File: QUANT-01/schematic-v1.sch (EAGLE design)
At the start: 1 part, among them U1 MCP4725

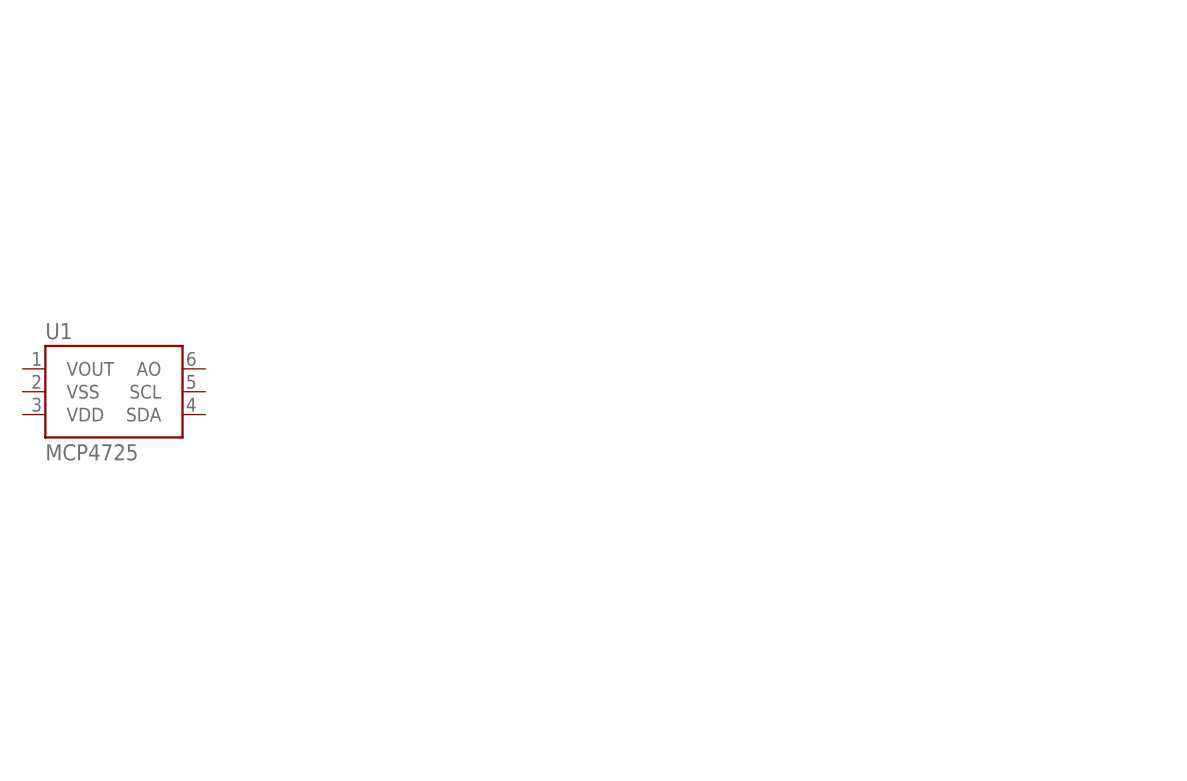
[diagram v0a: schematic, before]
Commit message: kind of got the quantization of Vin working.
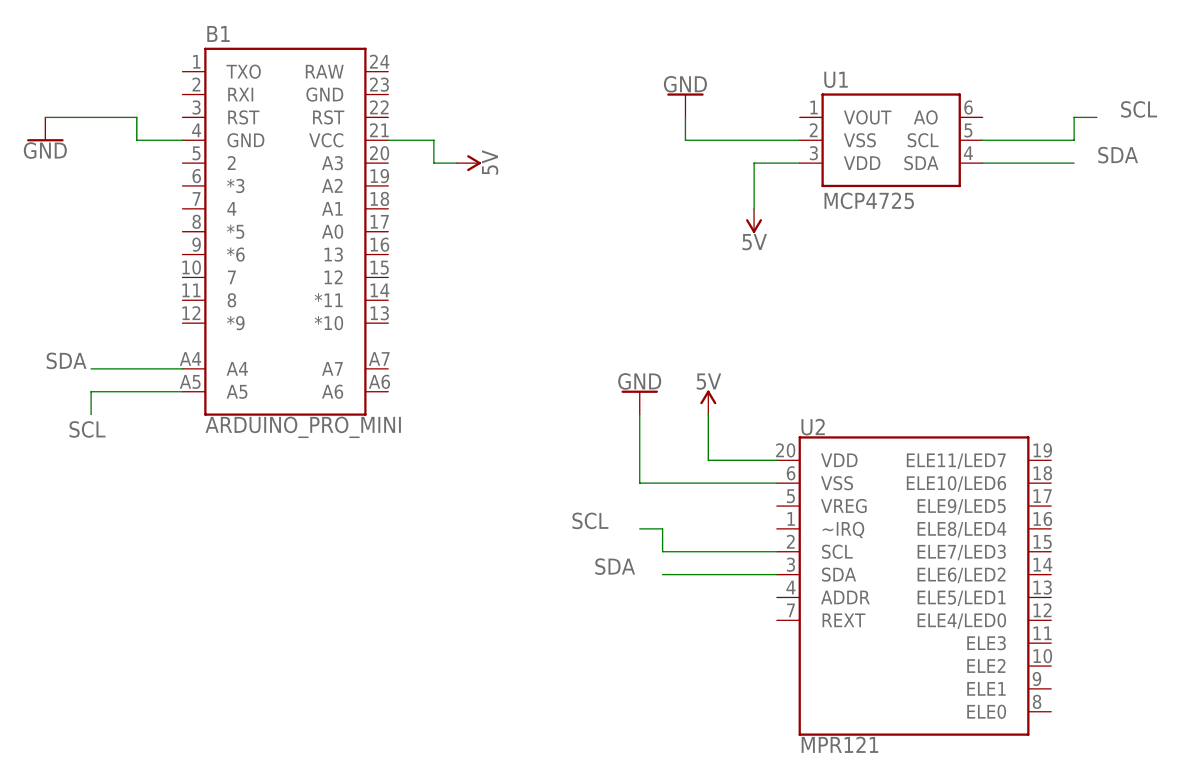
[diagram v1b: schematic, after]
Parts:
- added B1: ARDUINO_PRO_MINI, SparkFun-Boards:ARDUINO_PRO_MINI
- added U2: MPR121, SparkFun-Sensors:MPR121
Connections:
- new net 5V: B1.VCC, U1.VDD, U2.VDD
- new net GND: B1.GND, U1.VSS, U2.VSS
- new net SCL: B1.A5, U1.SCL, U2.SCL
- new net SDA: B1.A4, U1.SDA, U2.SDA
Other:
- moved on the sheet: U1
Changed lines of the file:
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@@
 <layer number="230" name="230bmp" color="7" fill="1" visible="yes" active="yes"/>
 <layer number="231" name="231bmp" color="7" fill="1" visible="yes" active="yes"/>
+<layer number="232" name="Eagle3D_PG2" color="7" fill="1" visible="yes" active="yes"/>
+<layer number="233" name="Eagle3D_PG3" color="7" fill="1" visible="yes" active="yes"/>
 <layer number="248" name="Housing" color="7" fill="1" visible="yes" active="yes"/>
 <layer number="249" name="Edge" color="7" fill="1" visible="yes" active="yes"/>
@@
 <parts>
 <part name="U1" library="SparkFun-IC-Conversion" library_urn="urn:adsk.eagle:library:522" deviceset="MCP4725" device="SOT-23" package3d_urn="urn:adsk.eagle:package:38775/1" value="MCP4725"/>
+<part name="U2" library="SparkFun-Sensors" deviceset="MPR121" device=""/>
+<part name="B1" library="SparkFun-Boards" library_urn="urn:adsk.eagle:library:509" deviceset="ARDUINO_PRO_MINI" device="" package3d_urn="urn:adsk.eagle:package:37322/1"/>
+<part name="GND1" library="SparkFun-PowerSymbols" library_urn="urn:adsk.eagle:library:530" deviceset="GND" device=""/>
+<part name="GND" library="SparkFun-PowerSymbols" library_urn="urn:adsk.eagle:library:530" deviceset="GND" device=""/>
+<part name="GND3" library="SparkFun-PowerSymbols" library_urn="urn:adsk.eagle:library:530" deviceset="GND" device=""/>
+<part name="SUPPLY1" library="SparkFun-PowerSymbols" library_urn="urn:adsk.eagle:library:530" deviceset="5V" device=""/>
+<part name="SUPPLY2" library="SparkFun-PowerSymbols" library_urn="urn:adsk.eagle:library:530" deviceset="5V" device=""/>
+<part name="SUPPLY3" library="SparkFun-PowerSymbols" library_urn="urn:adsk.eagle:library:530" deviceset="5V" device=""/>
 </parts>
 <sheets>
@@
 </plain>
 <instances>
-<instance part="U1" gate="U1" x="73.66" y="53.34"/>
+<instance part="U1" gate="U1" x="160.02" y="81.28"/>
+<instance part="U2" gate="G$1" x="162.56" y="33.02"/>
+<instance part="B1" gate="G$1" x="91.44" y="71.12"/>
+<instance part="GND1" gate="1" x="137.16" y="86.36" rot="R180"/>
+<instance part="GND" gate="1" x="66.04" y="81.28"/>
+<instance part="GND3" gate="1" x="132.08" y="53.34" rot="R180"/>
+<instance part="SUPPLY1" gate="G$1" x="111.76" y="78.74" rot="R270"/>
+<instance part="SUPPLY2" gate="G$1" x="144.78" y="73.66" rot="R180"/>
+<instance part="SUPPLY3" gate="G$1" x="139.7" y="50.8"/>
 </instances>
 <busses>
 </busses>
 <nets>
+<net name="SDA" class="0">
+<segment>
+<pinref part="U1" gate="U1" pin="SDA"/>
+<wire x1="170.18" y1="78.74" x2="180.34" y2="78.74" width="0.1524" layer="91"/>
+<label x="182.88" y="78.74" size="1.778" layer="95"/>
+</segment>
+<segment>
+<pinref part="U2" gate="G$1" pin="SDA"/>
+<wire x1="147.32" y1="33.02" x2="134.62" y2="33.02" width="0.1524" layer="91"/>
+<label x="127" y="33.02" size="1.778" layer="95"/>
+</segment>
+<segment>
+<pinref part="B1" gate="G$1" pin="A4"/>
+<wire x1="81.28" y1="55.88" x2="71.12" y2="55.88" width="0.1524" layer="91"/>
+<label x="66.04" y="55.88" size="1.778" layer="95"/>
+</segment>
+</net>
+<net name="SCL" class="0">
+<segment>
+<pinref part="B1" gate="G$1" pin="A5"/>
+<wire x1="81.28" y1="53.34" x2="71.12" y2="53.34" width="0.1524" layer="91"/>
+<wire x1="71.12" y1="53.34" x2="71.12" y2="50.8" width="0.1524" layer="91"/>
+<label x="68.58" y="48.26" size="1.778" layer="95"/>
+</segment>
+<segment>
+<pinref part="U2" gate="G$1" pin="SCL"/>
+<wire x1="147.32" y1="35.56" x2="134.62" y2="35.56" width="0.1524" layer="91"/>
+<wire x1="134.62" y1="35.56" x2="134.62" y2="38.1" width="0.1524" layer="91"/>
+<wire x1="134.62" y1="38.1" x2="132.08" y2="38.1" width="0.1524" layer="91"/>
+<label x="124.46" y="38.1" size="1.778" layer="95"/>
+</segment>
+<segment>
+<pinref part="U1" gate="U1" pin="SCL"/>
+<wire x1="170.18" y1="81.28" x2="180.34" y2="81.28" width="0.1524" layer="91"/>
+<wire x1="180.34" y1="81.28" x2="180.34" y2="83.82" width="0.1524" layer="91"/>
+<wire x1="180.34" y1="83.82" x2="182.88" y2="83.82" width="0.1524" layer="91"/>
+<label x="185.42" y="83.82" size="1.778" layer="95"/>
+</segment>
+</net>
+<net name="5V" class="0">
+<segment>
+<pinref part="U1" gate="U1" pin="VDD"/>
+<wire x1="149.86" y1="78.74" x2="144.78" y2="78.74" width="0.1524" layer="91"/>
+<pinref part="SUPPLY2" gate="G$1" pin="5V"/>
+<wire x1="144.78" y1="78.74" x2="144.78" y2="73.66" width="0.1524" layer="91"/>
+</segment>
+<segment>
+<pinref part="B1" gate="G$1" pin="VCC"/>
+<wire x1="104.14" y1="81.28" x2="109.22" y2="81.28" width="0.1524" layer="91"/>
+<wire x1="109.22" y1="81.28" x2="109.22" y2="78.74" width="0.1524" layer="91"/>
+<pinref part="SUPPLY1" gate="G$1" pin="5V"/>
+<wire x1="109.22" y1="78.74" x2="111.76" y2="78.74" width="0.1524" layer="91"/>
+</segment>
+<segment>
+<pinref part="U2" gate="G$1" pin="VDD"/>
+<wire x1="147.32" y1="45.72" x2="139.7" y2="45.72" width="0.1524" layer="91"/>
+<pinref part="SUPPLY3" gate="G$1" pin="5V"/>
+<wire x1="139.7" y1="45.72" x2="139.7" y2="50.8" width="0.1524" layer="91"/>
+</segment>
+</net>
+<net name="GND" class="0">
+<segment>
+<pinref part="U1" gate="U1" pin="VSS"/>
+<wire x1="149.86" y1="81.28" x2="137.16" y2="81.28" width="0.1524" layer="91"/>
+<pinref part="GND1" gate="1" pin="GND"/>
+<wire x1="137.16" y1="81.28" x2="137.16" y2="83.82" width="0.1524" layer="91"/>
+</segment>
+<segment>
+<pinref part="GND" gate="1" pin="GND"/>
+<wire x1="66.04" y1="83.82" x2="76.2" y2="83.82" width="0.1524" layer="91"/>
+<wire x1="76.2" y1="83.82" x2="76.2" y2="81.28" width="0.1524" layer="91"/>
+<pinref part="B1" gate="G$1" pin="GND"/>
+<wire x1="76.2" y1="81.28" x2="81.28" y2="81.28" width="0.1524" layer="91"/>
+</segment>
+<segment>
+<pinref part="U2" gate="G$1" pin="VSS"/>
+<wire x1="147.32" y1="43.18" x2="132.08" y2="43.18" width="0.1524" layer="91"/>
+<pinref part="GND3" gate="1" pin="GND"/>
+<wire x1="132.08" y1="43.18" x2="132.08" y2="50.8" width="0.1524" layer="91"/>
+</segment>
+</net>
 </nets>
 </sheet>
